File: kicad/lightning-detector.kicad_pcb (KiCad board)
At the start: 2 copper layers, 109.5 x 78.5 mm, 12 parts, among them J1 PWR, J3 Conn_01x03, U1 TFT_320x240, U3 TPS61023DRLR

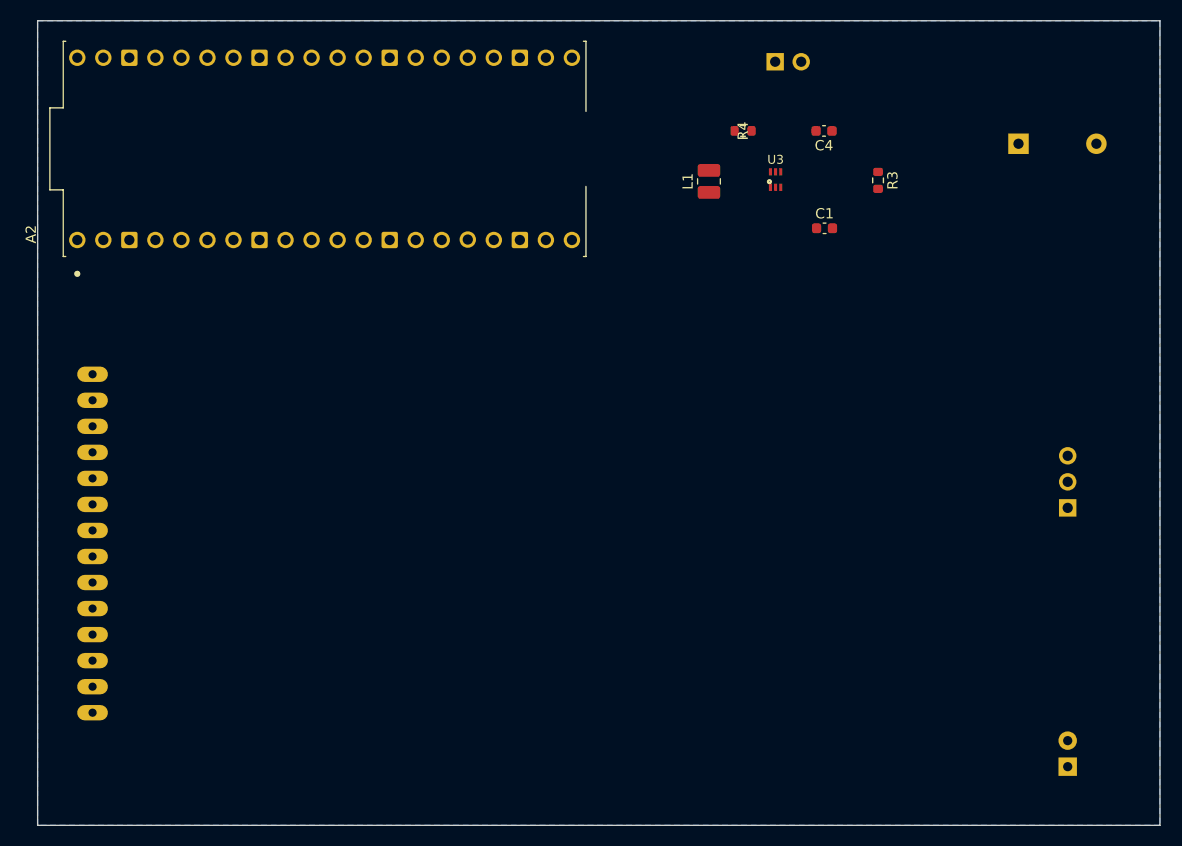
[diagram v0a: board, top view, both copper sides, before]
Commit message: wk07 items
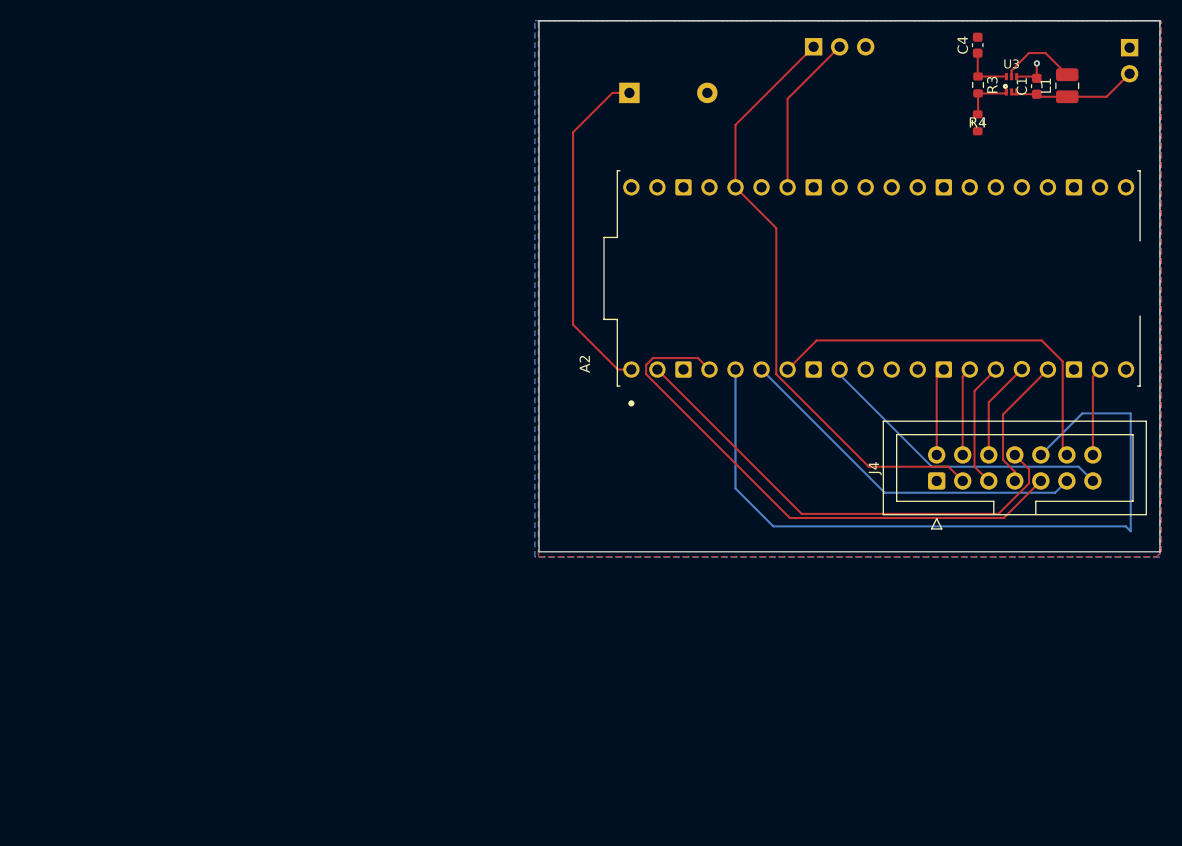
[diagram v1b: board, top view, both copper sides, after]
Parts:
- removed D1: LED, LED_THT:LED_D3.0mm
- removed U1: TFT_320x240, 3rdparty:TFT-320x240
- added J4: ADF7020 Breakout, Connector_IDC:IDC-Header_2x07_P2.54mm_Vertical, F.Cu at (182.7, 109.9)
- moved A2 55.5 mm to (177.1, 90.1)
- moved J3 51.4 mm to (170.7, 67.5), turned to -90 degrees
- moved BZ1 38.3 mm to (152.7, 72.0)
- moved L1 36.2 mm to (195.5, 71.3)
- moved J1 34.6 mm to (201.5, 67.6), turned to 180 degrees
- moved C1 24.9 mm to (192.5, 71.4), turned to 90 degrees
- moved U3 24.8 mm to (190.0, 71.2)
- moved R4 22.9 mm to (186.7, 75.0), turned to -90 degrees
- moved C4 17.2 mm to (186.7, 67.4), turned to 90 degrees
- moved R3 13.5 mm to (186.8, 71.3)
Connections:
- A2 pad 14: Net-(A2-GP10) -> /CLKOUT
- A2 pad 15: Net-(A2-GP11) -> /TXRXCLK
- A2 pad 16: Net-(A2-GP12) -> /TXRXDATA
- A2 pad 17: Net-(A2-GP13) -> /SWD_INT
- A2 pad 19: Net-(A2-GP14) -> /CE_70XX
- A2 pad 2: unconnected-(A2-GP1-Pad2) -> /ADC_IP
- A2 pad 20: Net-(A2-GP15) -> unconnected-(A2-GP15-Pad20)
- A2 pad 4: unconnected-(A2-GP2-Pad4) -> /SCLK
- A2 pad 5: unconnected-(A2-GP3-Pad5) -> /SREAD
- A2 pad 6: unconnected-(A2-GP4-Pad6) -> /SDATA
- A2 pad 7: unconnected-(A2-GP5-Pad7) -> /SLE
- A2 pad 9: unconnected-(A2-GP6-Pad9) -> /MUXOUT
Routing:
- net /SREAD: track 0.00 -> 73.8 mm
- net +3V3: track 0.00 -> 59.3 mm
- net /SCLK: track 0.00 -> 53.6 mm
- net /ADC_IP: track 0.00 -> 46.7 mm
- net /SLE: track 0.00 -> 38.2 mm
- net /SDATA: track 0.00 -> 35.2 mm
- net Net-(A2-GP0): track 0.00 -> 33.4 mm
- net /MUXOUT: track 0.00 -> 29.5 mm
- net /ADC_IN: track 0.00 -> 15.8 mm
- net /SWD_INT: track 0.00 -> 13.2 mm
- net +BATT: track 0.00 -> 12.6 mm
- net /TXRXCLK: track 0.00 -> 12.3 mm
- net GND: track 0.00 -> 12.1 mm, vias 0 -> 1
- net /TXRXDATA: track 0.00 -> 9.71 mm
- net /CLKOUT: track 0.00 -> 8.62 mm
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- added copper zone on F.Cu, net GND
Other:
- board size 109.5 x 78.5 mm -> 60.6 x 51.8 mm
